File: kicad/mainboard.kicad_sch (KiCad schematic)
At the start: 1 part, among them U1 4051

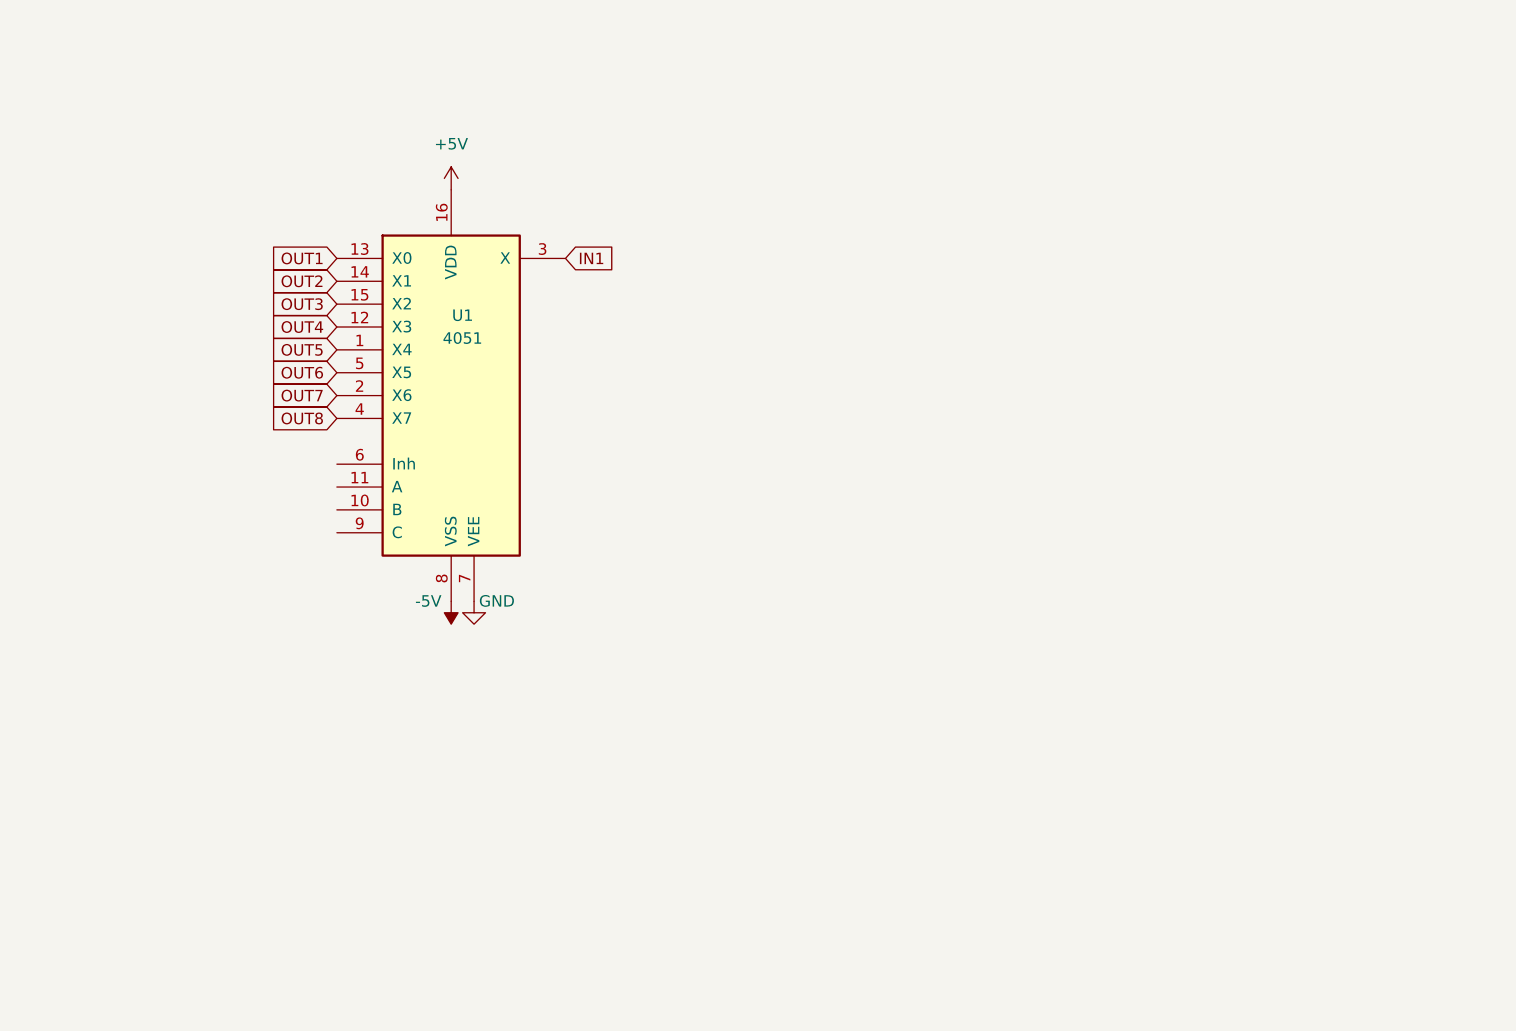
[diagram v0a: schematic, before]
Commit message: Added all 5041
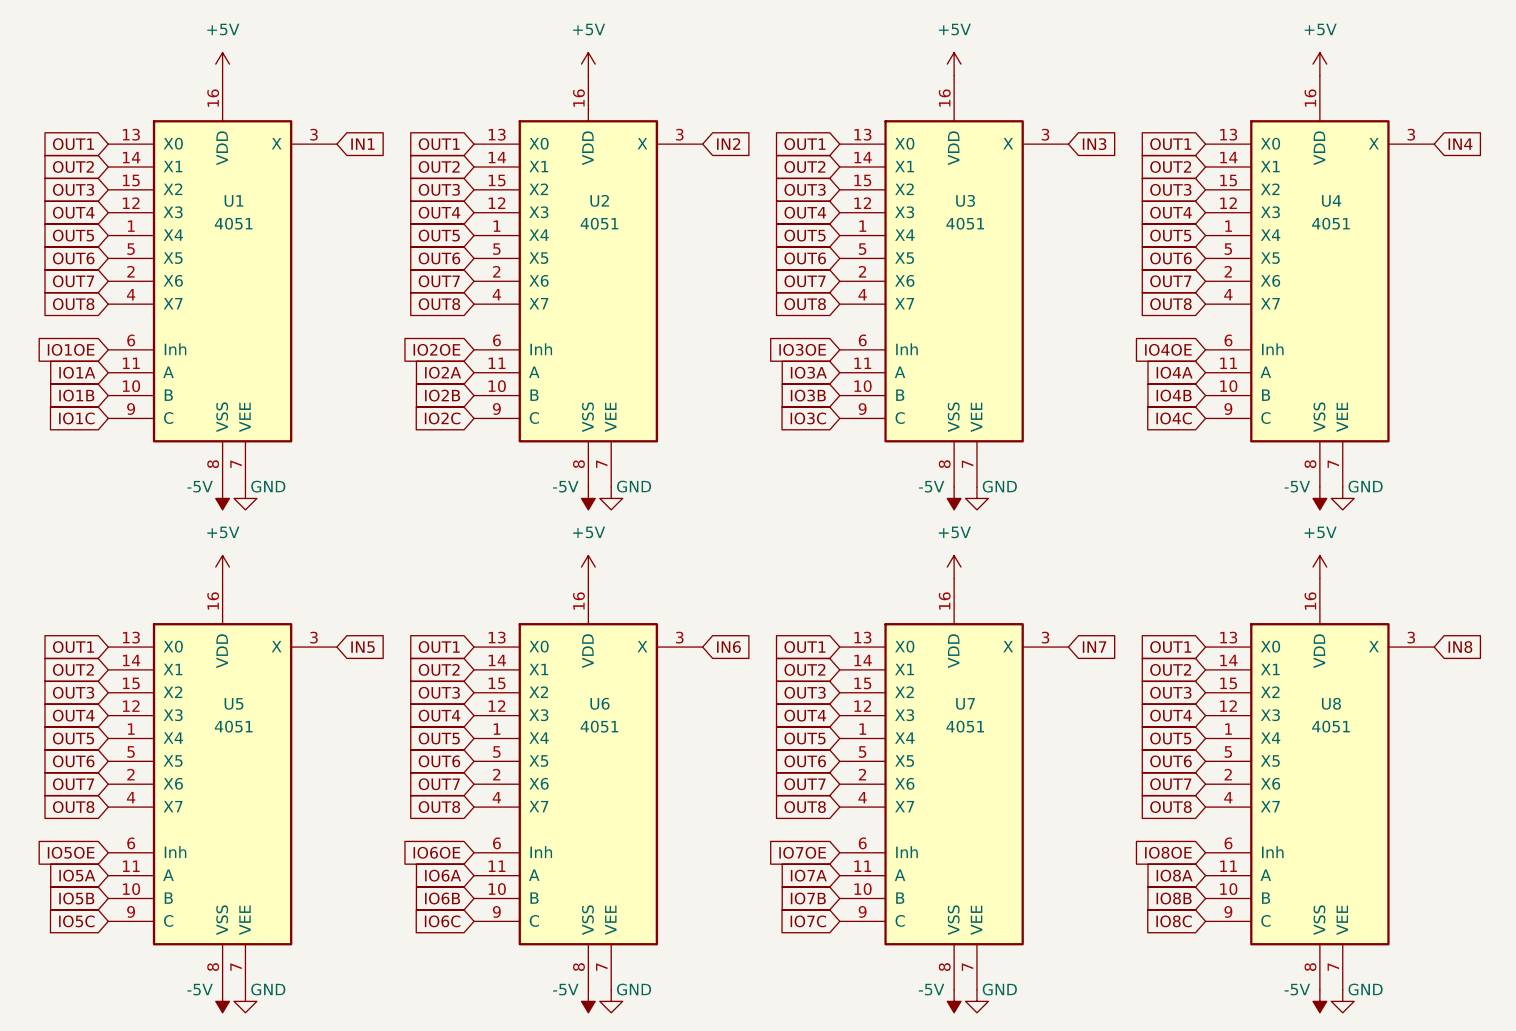
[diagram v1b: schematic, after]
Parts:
- added U2, U3, U4, U5, U6, U7, U8: 4051, symbol 4xxx:4051
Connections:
- net +5V: now also U2.16 (VDD), U3.16 (VDD), U4.16 (VDD), U5.16 (VDD), U6.16 (VDD), U7.16 (VDD), U8.16 (VDD)
- net -5V: now also U2.8 (VSS), U3.8 (VSS), U4.8 (VSS), U5.8 (VSS), U6.8 (VSS), U7.8 (VSS), U8.8 (VSS)
- net GND: now also U2.7 (VEE), U3.7 (VEE), U4.7 (VEE), U5.7 (VEE), U6.7 (VEE), U7.7 (VEE), U8.7 (VEE)
- net OUT1: now also U2.13 (X0), U3.13 (X0), U4.13 (X0), U5.13 (X0), U6.13 (X0), U7.13 (X0), U8.13 (X0)
- net OUT2: now also U2.14 (X1), U3.14 (X1), U4.14 (X1), U5.14 (X1), U6.14 (X1), U7.14 (X1), U8.14 (X1)
- net OUT3: now also U2.15 (X2), U3.15 (X2), U4.15 (X2), U5.15 (X2), U6.15 (X2), U7.15 (X2), U8.15 (X2)
- net OUT4: now also U2.12 (X3), U3.12 (X3), U4.12 (X3), U5.12 (X3), U6.12 (X3), U7.12 (X3), U8.12 (X3)
- net OUT5: now also U2.1 (X4), U3.1 (X4), U4.1 (X4), U5.1 (X4), U6.1 (X4), U7.1 (X4), U8.1 (X4)
- net OUT6: now also U2.5 (X5), U3.5 (X5), U4.5 (X5), U5.5 (X5), U6.5 (X5), U7.5 (X5), U8.5 (X5)
- net OUT7: now also U2.2 (X6), U3.2 (X6), U4.2 (X6), U5.2 (X6), U6.2 (X6), U7.2 (X6), U8.2 (X6)
- net OUT8: now also U2.4 (X7), U3.4 (X7), U4.4 (X7), U5.4 (X7), U6.4 (X7), U7.4 (X7), U8.4 (X7)
- net IO1B: now reaches U1.10 (B)
- net IO1A: now reaches U1.11 (A)
- net IO1OE: now reaches U1.6 (Inh)
- net IO1C: now reaches U1.9 (C)
- new net IN2: U2.3 (X)
- new net IN3: U3.3 (X)
- new net IN4: U4.3 (X)
- new net IN5: U5.3 (X)
- new net IN6: U6.3 (X)
- new net IN7: U7.3 (X)
- new net IN8: U8.3 (X)
- new net IO2A: U2.11 (A)
- new net IO2B: U2.10 (B)
- new net IO2C: U2.9 (C)
- new net IO2OE: U2.6 (Inh)
- new net IO3A: U3.11 (A)
- new net IO3B: U3.10 (B)
- new net IO3C: U3.9 (C)
- new net IO3OE: U3.6 (Inh)
- new net IO4A: U4.11 (A)
- new net IO4B: U4.10 (B)
- new net IO4C: U4.9 (C)
- new net IO4OE: U4.6 (Inh)
- new net IO5A: U5.11 (A)
- new net IO5B: U5.10 (B)
- new net IO5C: U5.9 (C)
- new net IO5OE: U5.6 (Inh)
- new net IO6A: U6.11 (A)
- new net IO6B: U6.10 (B)
- new net IO6C: U6.9 (C)
- new net IO6OE: U6.6 (Inh)
- new net IO7A: U7.11 (A)
- new net IO7B: U7.10 (B)
- new net IO7C: U7.9 (C)
- new net IO7OE: U7.6 (Inh)
- new net IO8A: U8.11 (A)
- new net IO8B: U8.10 (B)
- new net IO8C: U8.9 (C)
- new net IO8OE: U8.6 (Inh)
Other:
- moved on the sheet: U1
